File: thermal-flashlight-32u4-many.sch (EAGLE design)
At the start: 34 parts, among them IC2 MCP73831, IC3 ATMEGA32U4-AU, IC4 MCP1700-33, J1 AYZ0202, J2 1X2-3.5MM, Q4 BSS123, U1 MLX90614_, X1 USBSMD, X2 12MHz

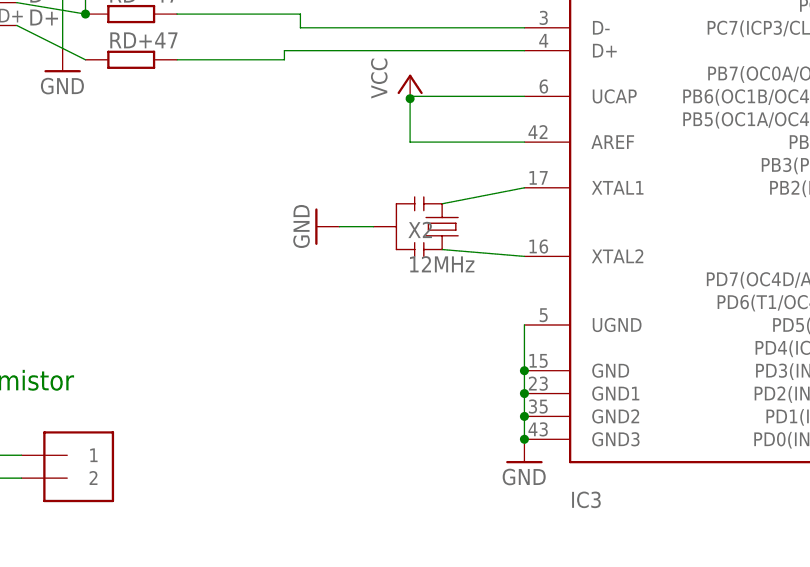
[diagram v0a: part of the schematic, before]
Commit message: update
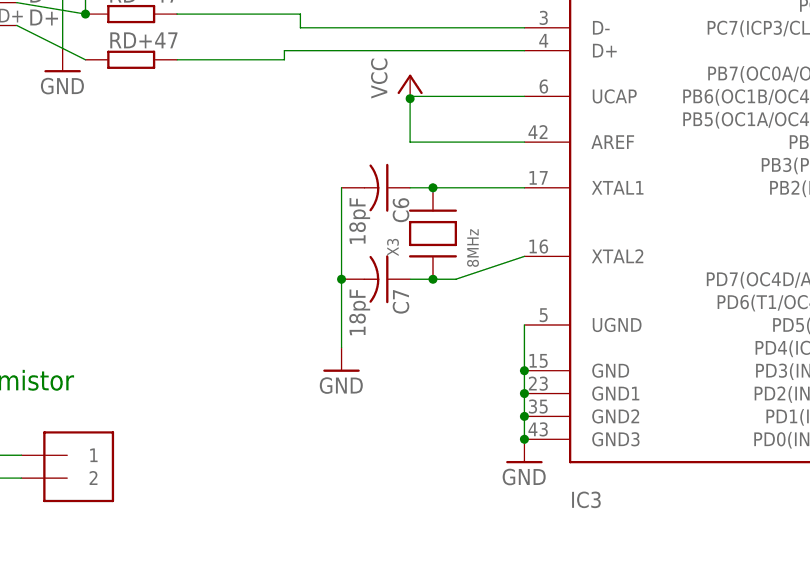
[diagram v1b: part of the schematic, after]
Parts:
- removed X2: 12MHz, SparkFunNew:RESONATORSMD
- added C6, C7: 18pF, adafruit:C-USC0805K
- added X3: 8MHz, adaprog:XTALNX5032
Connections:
- removed net N$22: X2.1
- removed net N$23: X2.3
- new net N$15: C7.1, IC3.XTAL2, X3.P$1
- new net N$16: C6.1, IC3.XTAL1, X3.P$2
- net GND: now also C6.2, C7.2; no longer X2.2
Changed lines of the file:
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@@
 </variantdefs>
 <classes>
-<class number="0" name="default" width="0.254" drill="0">
-<clearance class="0" value="0.2032"/>
+<class number="0" name="default" width="0" drill="0">
 </class>
 <class number="1" name="power" width="0.254" drill="0">
@@
 <part name="GND9" library="supply1" deviceset="GND" device=""/>
 <part name="GND10" library="supply1" deviceset="GND" device=""/>
+<part name="X3" library="adaprog" deviceset="XTAL" device="NX5032" value="8MHz"/>
+<part name="C6" library="adafruit" deviceset="C-US" device="C0805K" value="18pF"/>
+<part name="C7" library="adafruit" deviceset="C-US" device="C0805K" value="18pF"/>
 <part name="IC3" library="adaprog" deviceset="ATMEGA32U4" device="-AU"/>
 <part name="GND15" library="supply1" deviceset="GND" device=""/>
@@
 <part name="GND6" library="supply1" deviceset="GND" device=""/>
 <part name="RTHERM" library="rcl" deviceset="R-EU_" device="0204/7" value="330"/>
-<part name="X2" library="SparkFunNew" deviceset="RESONATOR" device="SMD" value="12MHz"/>
 </parts>
 <sheets>
@@
 <instance part="GND1" gate="1" x="-42.164" y="-58.42"/>
 <instance part="GND9" gate="1" x="19.812" y="-19.05"/>
-<instance part="GND10" gate="1" x="-3.302" y="7.112" rot="R270"/>
+<instance part="GND10" gate="1" x="-0.508" y="-8.89"/>
+<instance part="X3" gate="G$1" x="9.652" y="6.35" rot="R90"/>
+<instance part="C6" gate="G$1" x="4.572" y="11.43" rot="R270"/>
+<instance part="C7" gate="G$1" x="4.572" y="1.27" rot="R270"/>
 <instance part="IC3" gate="G$1" x="42.672" y="13.97"/>
 <instance part="GND15" gate="1" x="85.852" y="39.37" rot="MR270"/>
@@
 <instance part="RTHERM" gate="G$1" x="-42.164" y="-43.688" smashed="yes" rot="MR90">
 <attribute name="NAME" x="-29.972" y="-43.2054" size="1.778" layer="95" rot="MR0"/>
-</instance>
-<instance part="X2" gate="G$1" x="10.668" y="7.112" smashed="yes" rot="R270">
-<attribute name="NAME" x="6.858" y="5.842" size="1.778" layer="95"/>
-<attribute name="VALUE" x="6.858" y="2.032" size="1.778" layer="96"/>
 </instance>
 </instances>
@@
 </segment>
 <segment>
+<wire x1="-0.508" y1="-6.35" x2="-0.508" y2="1.27" width="0.1524" layer="91"/>
+<wire x1="-0.508" y1="11.43" x2="-0.508" y2="1.27" width="0.1524" layer="91"/>
+<junction x="-0.508" y="1.27"/>
+<pinref part="GND10" gate="1" pin="GND"/>
+<pinref part="C6" gate="G$1" pin="2"/>
+<pinref part="C7" gate="G$1" pin="2"/>
+</segment>
+<segment>
 <wire x1="83.312" y1="39.37" x2="68.072" y2="39.37" width="0.1524" layer="91"/>
 <pinref part="IC3" gate="G$1" pin="PE2(HWB)"/>
@@
 <junction x="274.32" y="25.4"/>
 <pinref part="GND6" gate="1" pin="GND"/>
-</segment>
-<segment>
-<pinref part="X2" gate="G$1" pin="2"/>
-<wire x1="3.048" y1="7.112" x2="-0.762" y2="7.112" width="0.1524" layer="91"/>
-<pinref part="GND10" gate="1" pin="GND"/>
 </segment>
 </net>
@@
 </segment>
 </net>
+<net name="N$15" class="0">
+<segment>
+<wire x1="19.812" y1="3.81" x2="12.192" y2="1.27" width="0.1524" layer="91"/>
+<wire x1="9.652" y1="1.27" x2="12.192" y2="1.27" width="0.1524" layer="91"/>
+<junction x="9.652" y="1.27"/>
+<pinref part="X3" gate="G$1" pin="P$1"/>
+<pinref part="C7" gate="G$1" pin="1"/>
+<pinref part="IC3" gate="G$1" pin="XTAL2"/>
+<wire x1="9.652" y1="1.27" x2="7.112" y2="1.27" width="0.1524" layer="91"/>
+</segment>
+</net>
+<net name="N$16" class="0">
+<segment>
+<wire x1="9.652" y1="11.43" x2="19.812" y2="11.43" width="0.1524" layer="91"/>
+<junction x="9.652" y="11.43"/>
+<pinref part="X3" gate="G$1" pin="P$2"/>
+<pinref part="C6" gate="G$1" pin="1"/>
+<pinref part="IC3" gate="G$1" pin="XTAL1"/>
+<wire x1="9.652" y1="11.43" x2="7.112" y2="11.43" width="0.1524" layer="91"/>
+</segment>
+</net>
 <net name="PC6" class="0">
 <segment>
@@
 </segment>
 </net>
-<net name="N$22" class="0">
-<segment>
-<pinref part="X2" gate="G$1" pin="1"/>
-<wire x1="10.668" y1="9.652" x2="19.812" y2="11.43" width="0.1524" layer="91"/>
-</segment>
-</net>
-<net name="N$23" class="0">
-<segment>
-<pinref part="X2" gate="G$1" pin="3"/>
-<wire x1="10.668" y1="4.572" x2="19.812" y2="3.81" width="0.1524" layer="91"/>
-</segment>
-</net>

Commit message: update
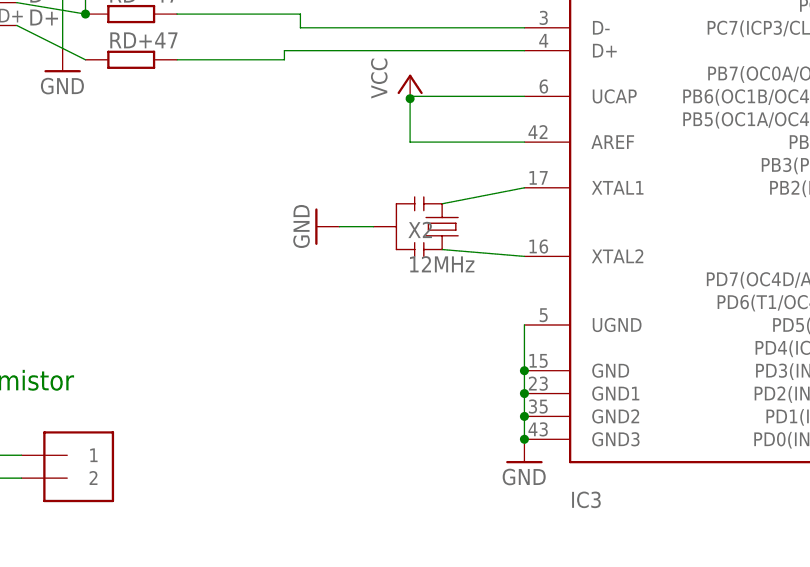
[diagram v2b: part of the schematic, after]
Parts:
- removed C6, C7: 18pF, adafruit:C-USC0805K
- removed X3: 8MHz, adaprog:XTALNX5032
- added X2: 12MHz, SparkFunNew:RESONATORSMD
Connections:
- removed net N$15: C7.1, IC3.XTAL2, X3.P$1
- removed net N$16: C6.1, IC3.XTAL1, X3.P$2
- new net N$22: X2.1
- new net N$23: X2.3
- net GND: now also X2.2; no longer C6.2, C7.2
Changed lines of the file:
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@@
 </variantdefs>
 <classes>
-<class number="0" name="default" width="0" drill="0">
+<class number="0" name="default" width="0.254" drill="0">
+<clearance class="0" value="0.2032"/>
 </class>
 <class number="1" name="power" width="0.254" drill="0">
@@
 <part name="GND9" library="supply1" deviceset="GND" device=""/>
 <part name="GND10" library="supply1" deviceset="GND" device=""/>
-<part name="X3" library="adaprog" deviceset="XTAL" device="NX5032" value="8MHz"/>
-<part name="C6" library="adafruit" deviceset="C-US" device="C0805K" value="18pF"/>
-<part name="C7" library="adafruit" deviceset="C-US" device="C0805K" value="18pF"/>
 <part name="IC3" library="adaprog" deviceset="ATMEGA32U4" device="-AU"/>
 <part name="GND15" library="supply1" deviceset="GND" device=""/>
@@
 <part name="GND6" library="supply1" deviceset="GND" device=""/>
 <part name="RTHERM" library="rcl" deviceset="R-EU_" device="0204/7" value="330"/>
+<part name="X2" library="SparkFunNew" deviceset="RESONATOR" device="SMD" value="12MHz"/>
 </parts>
 <sheets>
@@
 <instance part="GND1" gate="1" x="-42.164" y="-58.42"/>
 <instance part="GND9" gate="1" x="19.812" y="-19.05"/>
-<instance part="GND10" gate="1" x="-0.508" y="-8.89"/>
-<instance part="X3" gate="G$1" x="9.652" y="6.35" rot="R90"/>
-<instance part="C6" gate="G$1" x="4.572" y="11.43" rot="R270"/>
-<instance part="C7" gate="G$1" x="4.572" y="1.27" rot="R270"/>
+<instance part="GND10" gate="1" x="-3.302" y="7.112" rot="R270"/>
 <instance part="IC3" gate="G$1" x="42.672" y="13.97"/>
 <instance part="GND15" gate="1" x="85.852" y="39.37" rot="MR270"/>
@@
 <instance part="RTHERM" gate="G$1" x="-42.164" y="-43.688" smashed="yes" rot="MR90">
 <attribute name="NAME" x="-29.972" y="-43.2054" size="1.778" layer="95" rot="MR0"/>
+</instance>
+<instance part="X2" gate="G$1" x="10.668" y="7.112" smashed="yes" rot="R270">
+<attribute name="NAME" x="6.858" y="5.842" size="1.778" layer="95"/>
+<attribute name="VALUE" x="6.858" y="2.032" size="1.778" layer="96"/>
 </instance>
 </instances>
@@
 </segment>
 <segment>
-<wire x1="-0.508" y1="-6.35" x2="-0.508" y2="1.27" width="0.1524" layer="91"/>
-<wire x1="-0.508" y1="11.43" x2="-0.508" y2="1.27" width="0.1524" layer="91"/>
-<junction x="-0.508" y="1.27"/>
-<pinref part="GND10" gate="1" pin="GND"/>
-<pinref part="C6" gate="G$1" pin="2"/>
-<pinref part="C7" gate="G$1" pin="2"/>
-</segment>
-<segment>
 <wire x1="83.312" y1="39.37" x2="68.072" y2="39.37" width="0.1524" layer="91"/>
 <pinref part="IC3" gate="G$1" pin="PE2(HWB)"/>
@@
 <junction x="274.32" y="25.4"/>
 <pinref part="GND6" gate="1" pin="GND"/>
+</segment>
+<segment>
+<pinref part="X2" gate="G$1" pin="2"/>
+<wire x1="3.048" y1="7.112" x2="-0.762" y2="7.112" width="0.1524" layer="91"/>
+<pinref part="GND10" gate="1" pin="GND"/>
 </segment>
 </net>
@@
 </segment>
 </net>
-<net name="N$15" class="0">
-<segment>
-<wire x1="19.812" y1="3.81" x2="12.192" y2="1.27" width="0.1524" layer="91"/>
-<wire x1="9.652" y1="1.27" x2="12.192" y2="1.27" width="0.1524" layer="91"/>
-<junction x="9.652" y="1.27"/>
-<pinref part="X3" gate="G$1" pin="P$1"/>
-<pinref part="C7" gate="G$1" pin="1"/>
-<pinref part="IC3" gate="G$1" pin="XTAL2"/>
-<wire x1="9.652" y1="1.27" x2="7.112" y2="1.27" width="0.1524" layer="91"/>
-</segment>
-</net>
-<net name="N$16" class="0">
-<segment>
-<wire x1="9.652" y1="11.43" x2="19.812" y2="11.43" width="0.1524" layer="91"/>
-<junction x="9.652" y="11.43"/>
-<pinref part="X3" gate="G$1" pin="P$2"/>
-<pinref part="C6" gate="G$1" pin="1"/>
-<pinref part="IC3" gate="G$1" pin="XTAL1"/>
-<wire x1="9.652" y1="11.43" x2="7.112" y2="11.43" width="0.1524" layer="91"/>
-</segment>
-</net>
 <net name="PC6" class="0">
 <segment>
@@
 </segment>
 </net>
+<net name="N$22" class="0">
+<segment>
+<pinref part="X2" gate="G$1" pin="1"/>
+<wire x1="10.668" y1="9.652" x2="19.812" y2="11.43" width="0.1524" layer="91"/>
+</segment>
+</net>
+<net name="N$23" class="0">
+<segment>
+<pinref part="X2" gate="G$1" pin="3"/>
+<wire x1="10.668" y1="4.572" x2="19.812" y2="3.81" width="0.1524" layer="91"/>
+</segment>
+</net>
